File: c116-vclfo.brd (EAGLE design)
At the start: 100 x 50 mm, 66 parts, among them U1 SCREW-M2X8, U10 FX2-20S-1.27DS, U11 ERM1-5MM, U2 SCREW-M2X8, U3 NUT-M2-SELFLOCK, U4 NUT-M2-SELFLOCK, U5 FX2-20P-1.27DS, U6 SCREW-M2X8, U7 SCREW-M2X8, U8 NUT-M2-SELFLOCK, U9 NUT-M2-SELFLOCK

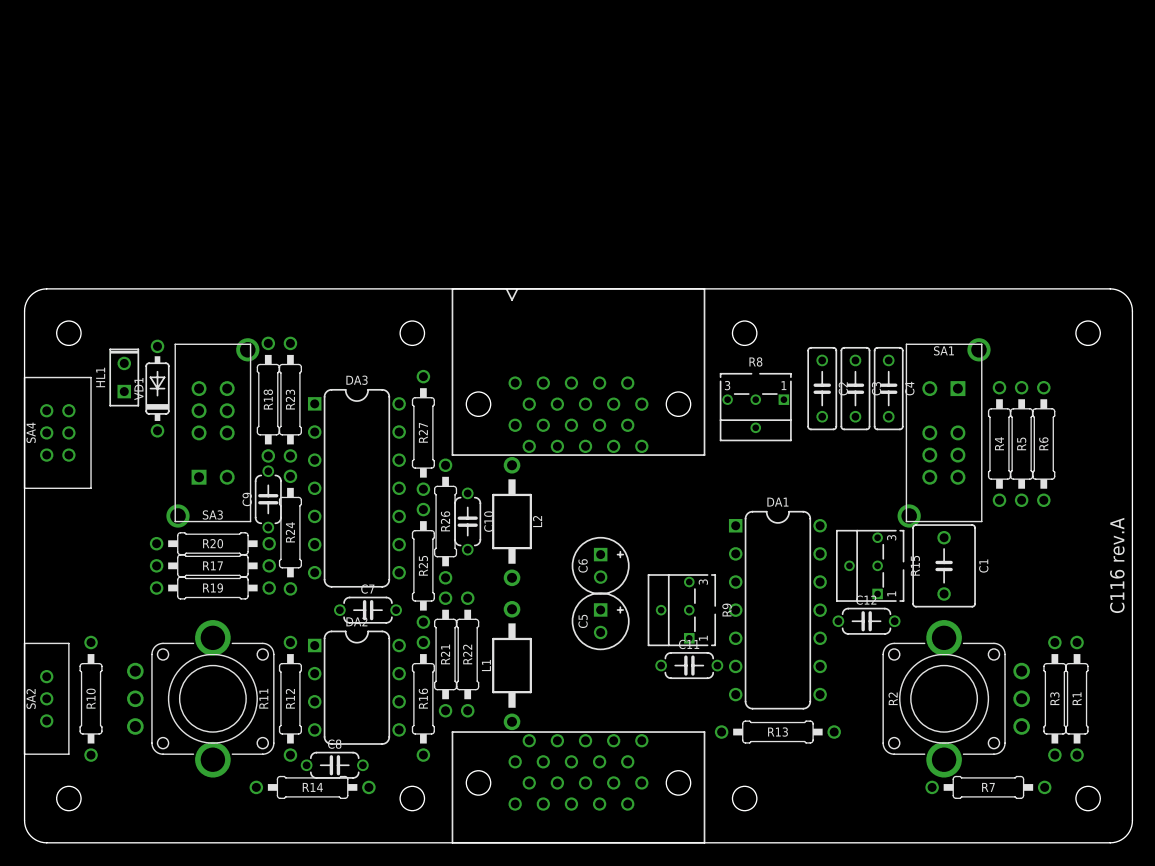
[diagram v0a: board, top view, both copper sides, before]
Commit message: C116 Update
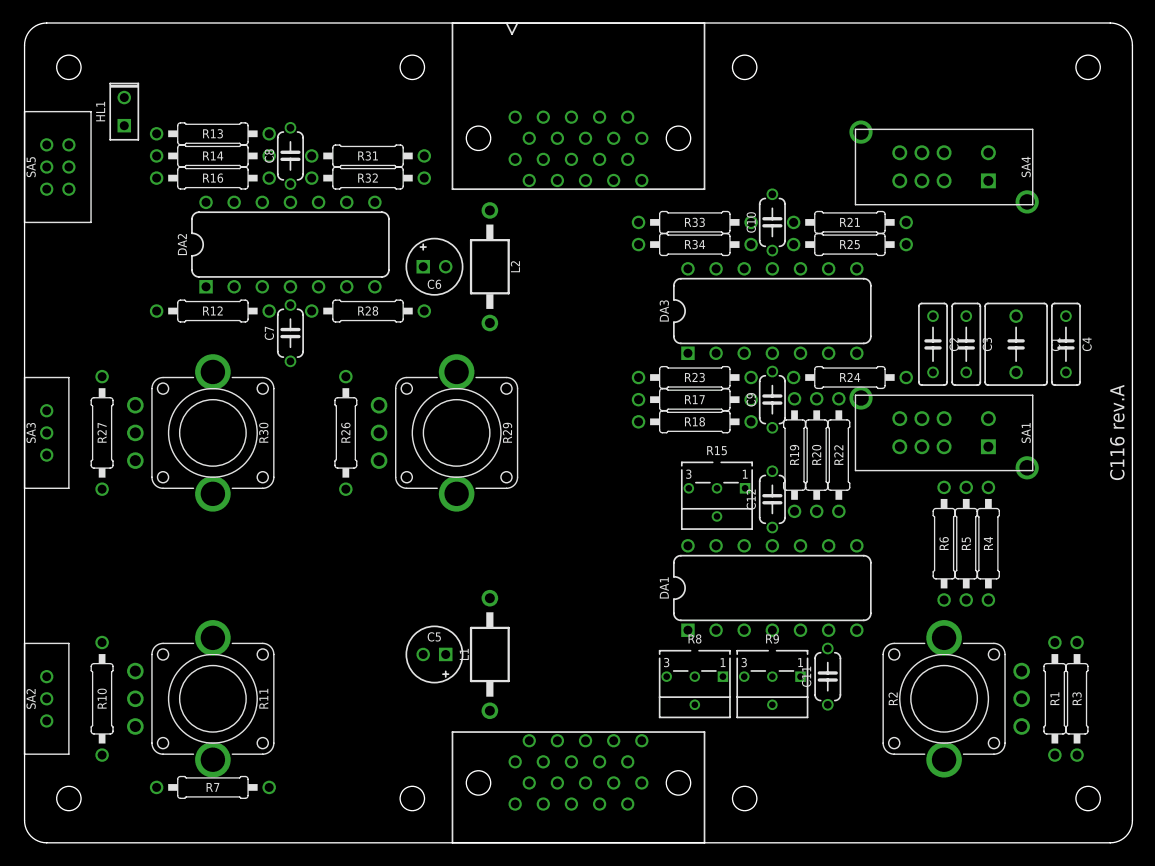
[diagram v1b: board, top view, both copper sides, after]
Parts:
- removed VD1: BAT46, diodes-schottky:DO35-7
- added O5, O7: 450-AA150(15MM,D,BLACK), hardware:EMPTY
- added O6, O8: 450-CP151(15MM,RED/WHITE), hardware:EMPTY
- added R28, R31, R32: 100K(TH), resistors:R-0207/10
- added R29, R30: B100K(CD)(9MM), potentiometers:RV09-SINGLE
- added R33, R34: 1K8(TH), resistors:R-0207/10
- added SA5: MJS22R, switches:APEM-MJS22R
- DA2: value TL072IP -> TL074CN; device ic-ti:DIP-8 -> ic-ti:DIP-14
- HL1: value YELLOW(2MMX5MM) -> RED/GREEN(2MMX5MM,BIPOLAR)
- PCB1: device module-footprints:ST2-BOARD-50 -> module-footprints:ST2-BOARD-74
- R26, R27: value 1K8(TH) -> 100K(TH)
- SA3: value MHS233K -> MJS12R; device switches:APEM-MHS233K -> switches:APEM-MJS12R
- SA4: value MJS22R -> MHS233K; device switches:APEM-MJS22R -> switches:APEM-MHS233K
- moved SA4 86.4 mm to (83.0, 61.0), turned to 180 degrees
- moved R13 74.3 mm to (17.0, 64.0)
- moved R7 70.0 mm to (17.0, 5.00)
- moved R14 57.7 mm to (17.0, 62.0)
- moved C8 55.1 mm to (24.0, 62.0), turned to 90 degrees
- moved R20 55.1 mm to (71.5, 35.0), turned to 90 degrees
- moved R19 53.9 mm to (69.5, 35.0), turned to 90 degrees
- moved R21 53.4 mm to (74.5, 56.0), turned to 180 degrees
- moved R24 52.4 mm to (74.5, 42.0), turned to 0 degrees
- moved R16 50.7 mm to (17.0, 60.0), turned to 180 degrees
- moved R25 48.2 mm to (74.5, 54.0), turned to 0 degrees
- moved C9 46.4 mm to (67.5, 40.0)
- moved R17 46.0 mm to (60.5, 40.0)
- moved U1 45.5 mm to (78.0, -127.0)
- moved U10 45.5 mm to (105.0, -127.0)
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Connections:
- removed net N$39: DA3.12, SA3.CMN, SA4.NC1, SA4.NO2
- new net N$37: R27.2, R30.2
- new net N$42: DA2.6, R28.1, R29.3, R30.3
- new net N$44: DA2.7, R28.2, R31.1
- new net N$45: DA2.9, R29.1, R30.1, R31.2, R32.1
- new net N$46: DA2.8, DA3.12, R32.2, SA5.NC1, SA5.NO2
- new net N$47: R27.1, SA3.C
- new net N$48: R26.2, R29.2
- new net N$49: R26.1, SA4.CMN
- net +15V: now also DA2.4; no longer DA2.8
- net -15V: now also DA2.11; no longer DA2.4
- net CV1_IN: now also SA3.NO, SA5.NC2; no longer SA4.NC2
- net CV1_OUT: now also SA5.C2; no longer SA4.C2
- net CV2_IN: now also SA3.NC, SA5.NO1; no longer SA4.NO1
- net CV2_OUT: now also SA5.C1; no longer SA4.C1
- net GND: now also DA2.10, DA2.12, R33.2; no longer R26.2
- net N$22: now also SA4.1; no longer SA3.1
- net N$29: now also SA4.2; no longer SA3.2
- net N$32: now also SA4.3; no longer SA3.3
- net N$36: now also R33.1, R34.2; no longer R26.1, R27.2
- net N$40: now also HL1.A, R34.1; no longer HL1.K, R27.1, VD1.A
- net N$41: now also HL1.K; no longer HL1.A, VD1.C
- net N$7: now also DA2.13; no longer DA2.6
- net N$8: now also DA2.14; no longer DA2.7
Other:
- board size 100 x 50 mm -> 100 x 74 mm
